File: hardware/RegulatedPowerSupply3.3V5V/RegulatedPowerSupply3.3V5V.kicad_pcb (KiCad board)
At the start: 2 copper layers, 80 x 50 mm, 11 parts, among them J1 Conn_01x04_Pin, J2 1x02 Pin, J3 1x02 Pin

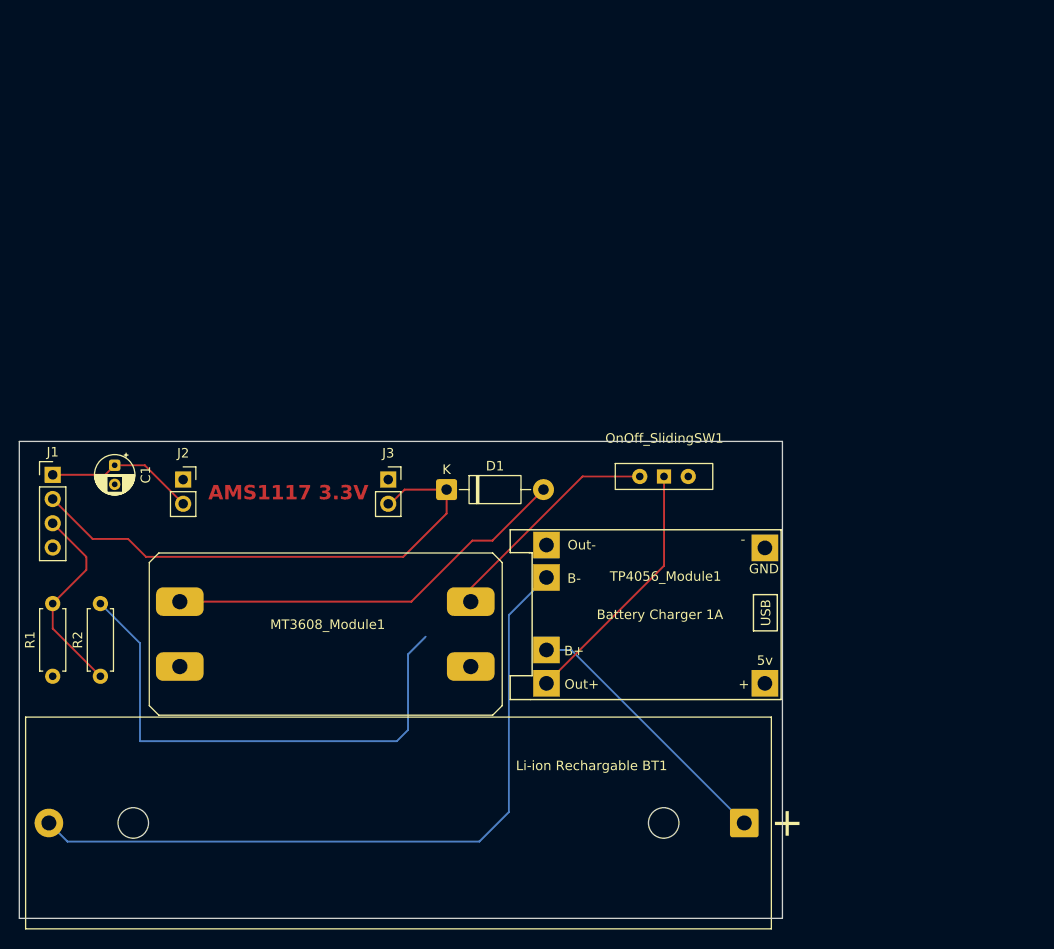
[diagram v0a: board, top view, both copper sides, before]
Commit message: KiCad
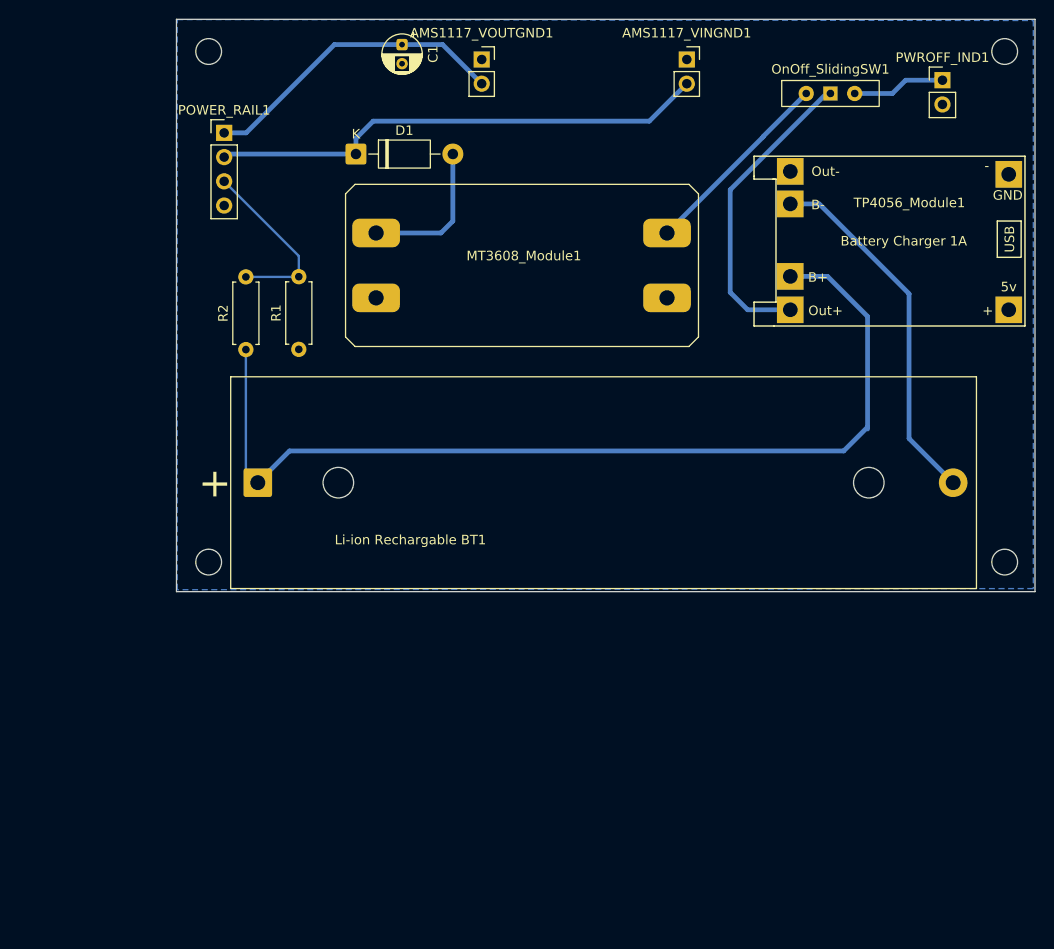
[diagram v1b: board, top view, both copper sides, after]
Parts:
- removed J2, J3: 1x02 Pin, Connector_PinSocket_2.54mm:PinSocket_1x02_P2.54mm_Vertical
- added AMS1117_VINGND1: 1x02 Pin, Connector_PinSocket_2.54mm:PinSocket_1x02_P2.54mm_Vertical, F.Cu at (151.0, 73.0)
- added AMS1117_VOUTGND1: 1x02 Pin, Connector_PinSocket_2.54mm:PinSocket_1x02_P2.54mm_Vertical, F.Cu at (129.5, 73.0)
- added PWROFF_IND1: Conn_01x02_Pin, Connector_PinHeader_2.54mm:PinHeader_1x02_P2.54mm_Vertical, F.Cu at (177.8, 75.1)
- added REF**: MountingHole_2.7mm_M2.5, MountingHole:MountingHole_2.7mm_M2.5, F.Cu at (184.3, 72.1)
- added REF**: MountingHole_2.7mm_M2.5, MountingHole:MountingHole_2.7mm_M2.5, F.Cu at (184.3, 125.7)
- added REF**: MountingHole_2.7mm_M2.5, MountingHole:MountingHole_2.7mm_M2.5, F.Cu at (100.8, 125.7)
- added REF**: MountingHole_2.7mm_M2.5, MountingHole:MountingHole_2.7mm_M2.5, F.Cu at (100.8, 72.1)
- POWER_RAIL1: renamed from J1; value Conn_01x04_Pin -> 1x04 PIN
- moved Li-ion Rechargable BT1 62.2 mm to (106.0, 117.3), turned to 0 degrees
- moved C1 53.4 mm to (121.1, 71.4)
- moved TP4056_Module1 46.8 mm to (186.4, 100.9)
- moved MT3608_Module1 43.8 mm to (133.9, 94.0)
- moved OnOff_SlidingSW1 43.8 mm to (166.0, 76.5)
- moved R1 42.9 mm to (110.3, 103.3)
- moved POWER_RAIL1 40.1 mm to (102.5, 80.7)
- moved R2 37.5 mm to (104.8, 103.4)
- moved D1 36.4 mm to (116.3, 82.9)
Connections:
- net Net-(Li-ion Rechargable BT1--) renamed /BATT-
- D1 pad 2: Net-(D1-A) -> /5V
- Li-ion Rechargable BT1 pad 1: Net-(Li-ion Rechargable BT1-+) -> /BATT+
- MT3608_Module1 pad 1: Net-(MT3608_Module1-VIN+) -> /TP4056+
- MT3608_Module1 pad 4: Net-(D1-A) -> /5V
- OnOff_SlidingSW1 pad 1: Net-(OnOff_SlidingSW1-B) -> /TP4056+
- OnOff_SlidingSW1 pad 2: Net-(MT3608_Module1-VIN+) -> /TP4056+
- OnOff_SlidingSW1 pad 3: unconnected-(OnOff_SlidingSW1-A-Pad3) -> Net-(OnOff_SlidingSW1-A)
- POWER_RAIL1 pad 3: /Battery_Sense -> /BATT+
- R1 pad 2: /Battery_Sense -> /BATT+
- R2 pad 1: /Battery_Sense -> /BATT+
- R2 pad 2: Net-(Li-ion Rechargable BT1-+) -> /BATT+
- TP4056_Module1 pad 3: Net-(OnOff_SlidingSW1-B) -> /TP4056+
- TP4056_Module1 pad 5: Net-(Li-ion Rechargable BT1-+) -> /BATT+
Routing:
- net /BATT+: track 0.00 -> 121.2 mm
- net Net-(Li-ion Rechargable BT1-+): track 83.5 -> 0.00 mm
- net /TP4056+: track 0.00 -> 53.2 mm
- net Net-(D1-A): track 43.0 -> 0.00 mm
- net /BATT-: track 76.5 -> 38.1 mm
- net Net-(OnOff_SlidingSW1-B): track 26.8 -> 0.00 mm
- net Net-(MT3608_Module1-VIN+): track 24.0 -> 0.00 mm
- net /Battery_Sense: track 21.0 -> 0.00 mm
- net /3.3V: track 15.8 -> 32.5 mm
- net /5V: track 54.6 -> 68.2 mm
- net Net-(OnOff_SlidingSW1-A): track 0.00 -> 9.78 mm
- added copper zone on B.Cu, net GND
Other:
- board size 80 x 50 mm -> 90 x 60 mm
- board text removed: "AMS1117 3.3V"
